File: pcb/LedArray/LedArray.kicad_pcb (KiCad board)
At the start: 2 copper layers, 49.8 x 49.8 mm, 422 parts

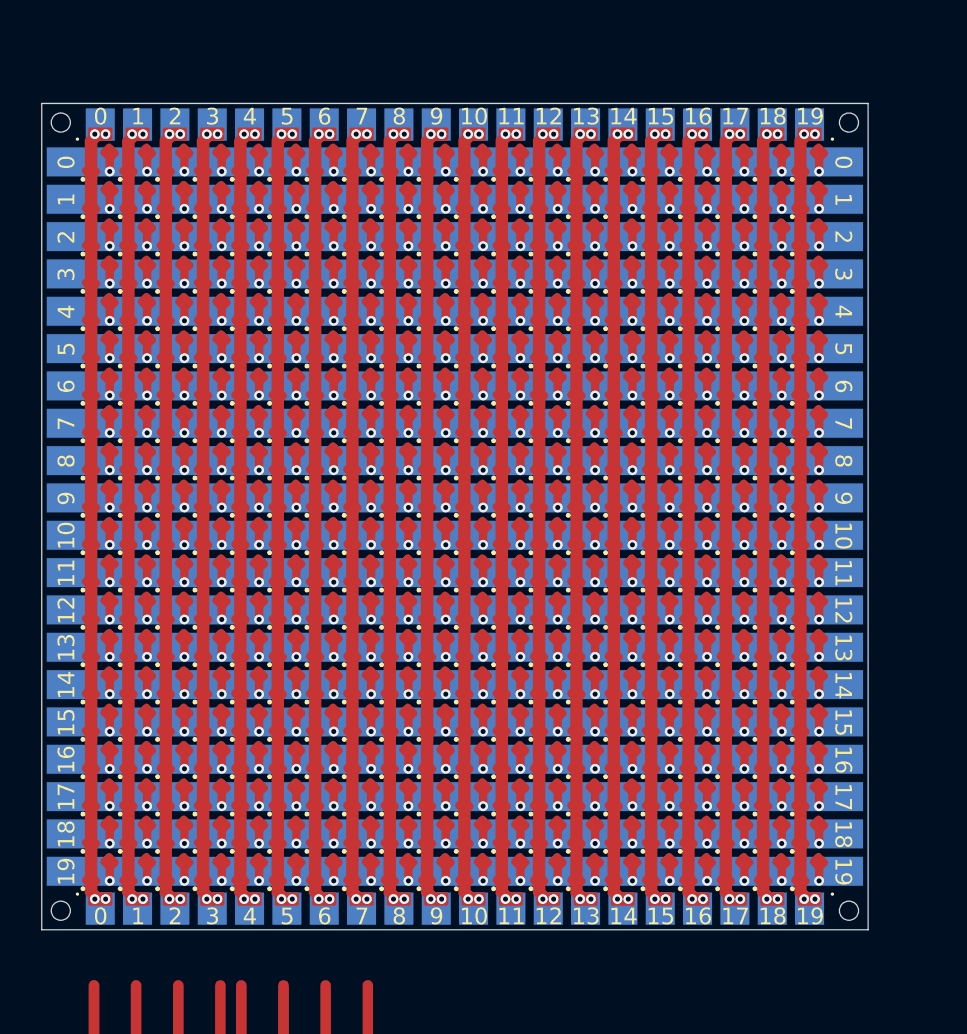
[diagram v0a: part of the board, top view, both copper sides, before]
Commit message: LedArray Rev B
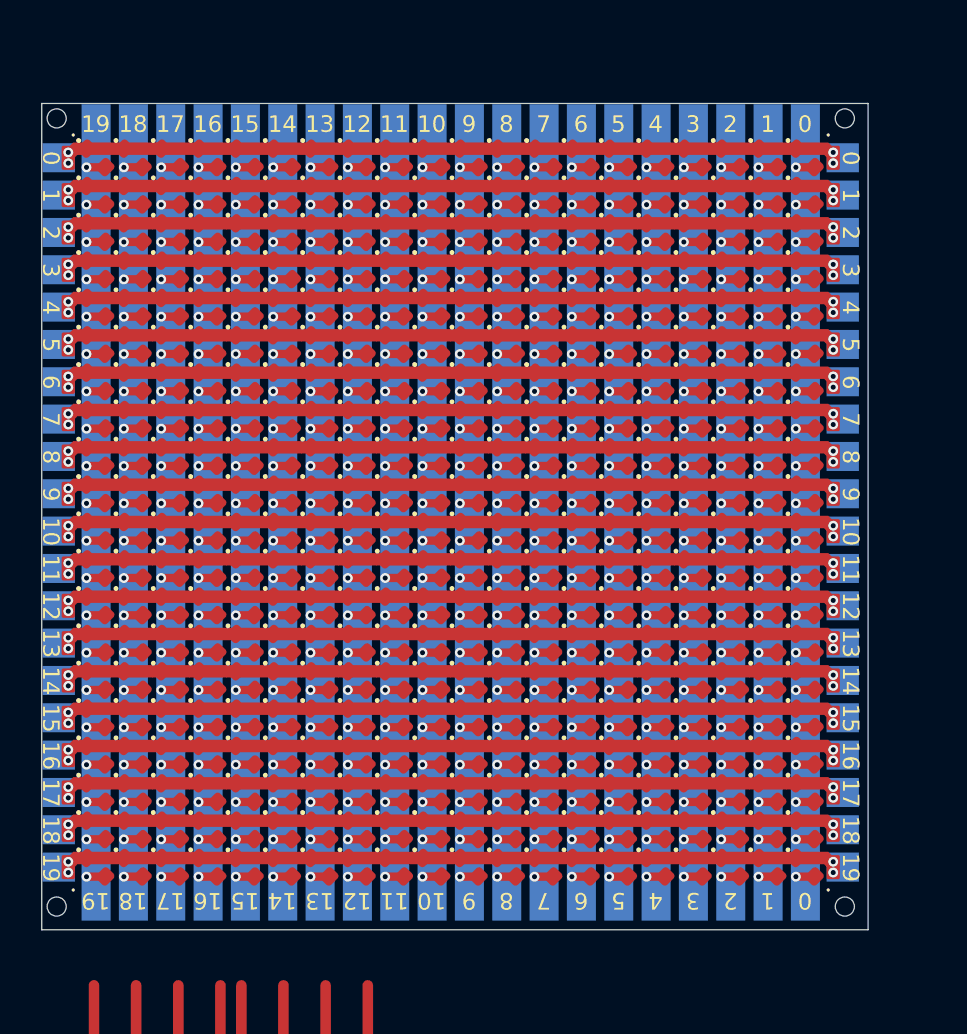
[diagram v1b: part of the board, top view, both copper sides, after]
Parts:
- moved ? 47.8 mm to (121.5, 89.0), turned to 180 degrees
- moved ? 47.8 mm to (121.5, 41.5), turned to 90 degrees
- moved ? 47.3 mm to (169.0, 41.5), turned to 0 degrees
- moved ? 47.3 mm to (169.0, 89.0), turned to -90 degrees
- moved D1 43.0 mm to (123.9, 86.6), turned to -45 degrees
- moved D1 43.0 mm to (123.9, 43.9), turned to -45 degrees
- moved D1 42.5 mm to (166.6, 86.6), turned to -45 degrees
- moved D1 42.5 mm to (166.6, 43.9), turned to -45 degrees
- moved D1 40.8 mm to (123.9, 84.4), turned to -45 degrees
- moved D1 40.8 mm to (123.9, 46.1), turned to -45 degrees
- moved D1 40.8 mm to (126.1, 86.6), turned to -45 degrees
- moved D1 40.8 mm to (126.1, 43.9), turned to -45 degrees
- moved D1 40.3 mm to (164.4, 86.6), turned to -45 degrees
- moved D1 40.3 mm to (164.4, 43.9), turned to -45 degrees
- moved D1 40.3 mm to (166.6, 84.4), turned to -45 degrees
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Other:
- board text added: "Forward voltage: 1.9-2.3 V at 20mA"
- board text added: "JLCJLCJLCJLC"
- board text added: "Max continuous current: 20mA"
- board text added: "Max peak current: 80mA"
- board text added: "Rev B"
- board text removed: "Current: 25mA"
- board text removed: "Forward voltage: 1.8V - 2.1 V"
- board text removed: "Max current: 70mA"
- board text removed: "Rev A"
